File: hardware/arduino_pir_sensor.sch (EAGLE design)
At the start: 44 parts, among them U2 TPS61097-33, U3 BISS0001SO16, U4 NRF24L01+_MODULE, U5 D203S

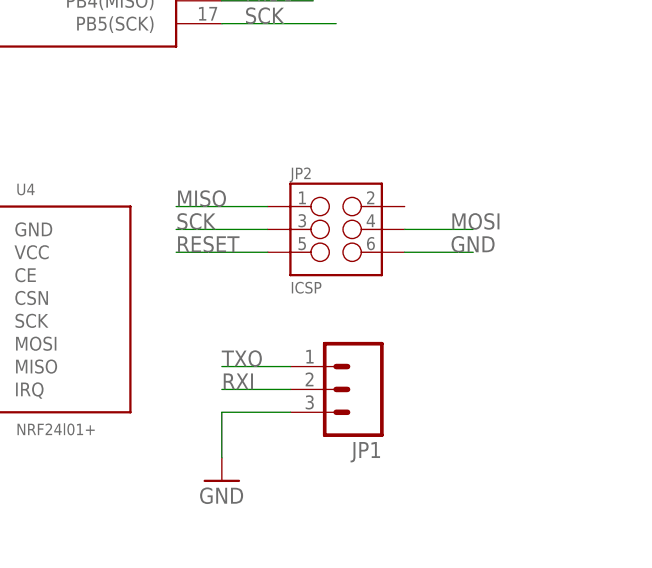
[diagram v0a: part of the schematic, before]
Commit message: - schematic pdf file updated
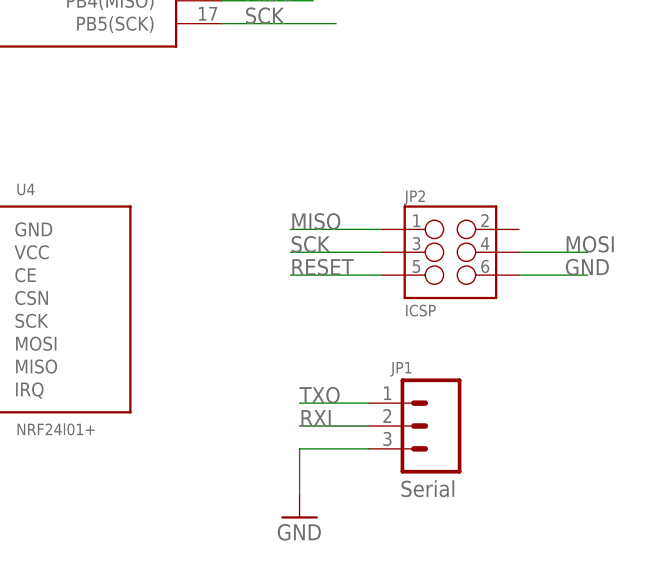
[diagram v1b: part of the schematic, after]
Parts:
- JP1: value (none) -> Serial
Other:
- moved on the sheet: JP1, JP2
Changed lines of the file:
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@@
 <part name="P+8" library="SparkFun" deviceset="3.3V" device="" value="VCC"/>
 <part name="FRAME1" library="SparkFun-Aesthetics" deviceset="FRAME-A3" device=""/>
-<part name="JP1" library="endy-connectors" deviceset="M03" device="PTH"/>
+<part name="JP1" library="endy-connectors" deviceset="M03" device="PTH" value="Serial"/>
 <part name="GND20" library="SparkFun" deviceset="GND" device=""/>
 </parts>
@@
 </instance>
 <instance part="P+3" gate="G$1" x="91.44" y="134.62"/>
-<instance part="JP2" gate="G$1" x="182.88" y="35.56">
-<attribute name="OC_NEWARK" x="182.88" y="35.56" size="1.778" layer="96" display="off"/>
-<attribute name="MF" x="182.88" y="35.56" size="1.778" layer="96" display="off"/>
-<attribute name="MPN" x="182.88" y="35.56" size="1.778" layer="96" display="off"/>
+<instance part="JP2" gate="G$1" x="195.58" y="33.02" smashed="yes">
+<attribute name="OC_NEWARK" x="195.58" y="33.02" size="1.778" layer="96" display="off"/>
+<attribute name="MF" x="195.58" y="33.02" size="1.778" layer="96" display="off"/>
+<attribute name="MPN" x="195.58" y="33.02" size="1.778" layer="96" display="off"/>
+<attribute name="NAME" x="190.5" y="38.608" size="1.27" layer="95"/>
+<attribute name="VALUE" x="190.5" y="25.908" size="1.27" layer="96"/>
 </instance>
 <instance part="C2" gate="G$1" x="93.98" y="63.5">
@@
 <instance part="P+8" gate="G$1" x="63.5" y="162.56"/>
 <instance part="FRAME1" gate="G$1" x="-142.24" y="-68.58"/>
-<instance part="JP1" gate="G$1" x="185.42" y="17.78" rot="R180"/>
-<instance part="GND20" gate="1" x="170.18" y="7.62"/>
+<instance part="JP1" gate="G$1" x="194.056" y="13.716" smashed="yes" rot="R180">
+<attribute name="VALUE" x="189.992" y="5.842" size="1.778" layer="96"/>
+<attribute name="NAME" x="188.976" y="19.558" size="1.27" layer="95"/>
+</instance>
+<instance part="GND20" gate="1" x="178.816" y="3.556"/>
 </instances>
 <busses>
@@
 <segment>
 <pinref part="JP2" gate="G$1" pin="6"/>
-<wire x1="198.12" y1="33.02" x2="190.5" y2="33.02" width="0.1524" layer="91"/>
-<label x="195.58" y="33.02" size="1.778" layer="95"/>
+<wire x1="210.82" y1="30.48" x2="203.2" y2="30.48" width="0.1524" layer="91"/>
+<label x="208.28" y="30.48" size="1.778" layer="95"/>
 </segment>
 <segment>
@@
 <pinref part="JP1" gate="G$1" pin="3"/>
 <pinref part="GND20" gate="1" pin="GND"/>
-<wire x1="177.8" y1="15.24" x2="170.18" y2="15.24" width="0.1524" layer="91"/>
-<wire x1="170.18" y1="15.24" x2="170.18" y2="10.16" width="0.1524" layer="91"/>
+<wire x1="186.436" y1="11.176" x2="178.816" y2="11.176" width="0.1524" layer="91"/>
+<wire x1="178.816" y1="11.176" x2="178.816" y2="6.096" width="0.1524" layer="91"/>
 </segment>
 </net>
@@
 <segment>
 <pinref part="JP2" gate="G$1" pin="5"/>
-<wire x1="165.1" y1="33.02" x2="175.26" y2="33.02" width="0.1524" layer="91"/>
-<label x="165.1" y="33.02" size="1.778" layer="95"/>
+<wire x1="177.8" y1="30.48" x2="187.96" y2="30.48" width="0.1524" layer="91"/>
+<label x="177.8" y="30.48" size="1.778" layer="95"/>
 </segment>
 </net>
@@
 <segment>
 <pinref part="JP2" gate="G$1" pin="3"/>
-<wire x1="165.1" y1="35.56" x2="175.26" y2="35.56" width="0.1524" layer="91"/>
-<label x="165.1" y="35.56" size="1.778" layer="95"/>
+<wire x1="177.8" y1="33.02" x2="187.96" y2="33.02" width="0.1524" layer="91"/>
+<label x="177.8" y="33.02" size="1.778" layer="95"/>
 </segment>
 </net>
@@
 <segment>
 <pinref part="JP2" gate="G$1" pin="1"/>
-<wire x1="165.1" y1="38.1" x2="175.26" y2="38.1" width="0.1524" layer="91"/>
-<label x="165.1" y="38.1" size="1.778" layer="95"/>
+<wire x1="177.8" y1="35.56" x2="187.96" y2="35.56" width="0.1524" layer="91"/>
+<label x="177.8" y="35.56" size="1.778" layer="95"/>
 </segment>
 </net>
@@
 <segment>
 <pinref part="JP2" gate="G$1" pin="4"/>
-<wire x1="198.12" y1="35.56" x2="190.5" y2="35.56" width="0.1524" layer="91"/>
-<label x="195.58" y="35.56" size="1.778" layer="95"/>
+<wire x1="210.82" y1="33.02" x2="203.2" y2="33.02" width="0.1524" layer="91"/>
+<label x="208.28" y="33.02" size="1.778" layer="95"/>
 </segment>
 </net>
@@
 <segment>
 <pinref part="JP1" gate="G$1" pin="1"/>
-<wire x1="177.8" y1="20.32" x2="170.18" y2="20.32" width="0.1524" layer="91"/>
-<label x="170.18" y="20.32" size="1.778" layer="95"/>
+<wire x1="186.436" y1="16.256" x2="178.816" y2="16.256" width="0.1524" layer="91"/>
+<label x="178.816" y="16.256" size="1.778" layer="95"/>
 </segment>
 </net>
@@
 <segment>
 <pinref part="JP1" gate="G$1" pin="2"/>
-<wire x1="177.8" y1="17.78" x2="170.18" y2="17.78" width="0.1524" layer="91"/>
-<label x="170.18" y="17.78" size="1.778" layer="95"/>
-</segment>
-</net>
+<wire x1="186.436" y1="13.716" x2="178.816" y2="13.716" width="0.1524" layer="91"/>
+<label x="178.816" y="13.716" size="1.778" layer="95"/>
+</segment>
+</net>
